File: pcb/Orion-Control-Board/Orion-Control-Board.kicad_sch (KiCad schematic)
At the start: 59 parts, among them J1 CONN_20_POS_KEYED_SOCKET, U1 BNO055, U2 INA3221, U3 DFR0753 5V BUCK, U4 PCA9685_PWM_SERVO_DRIVER_IC, U5 INA3221, U6 INA3221, Y1 32.768 kHz

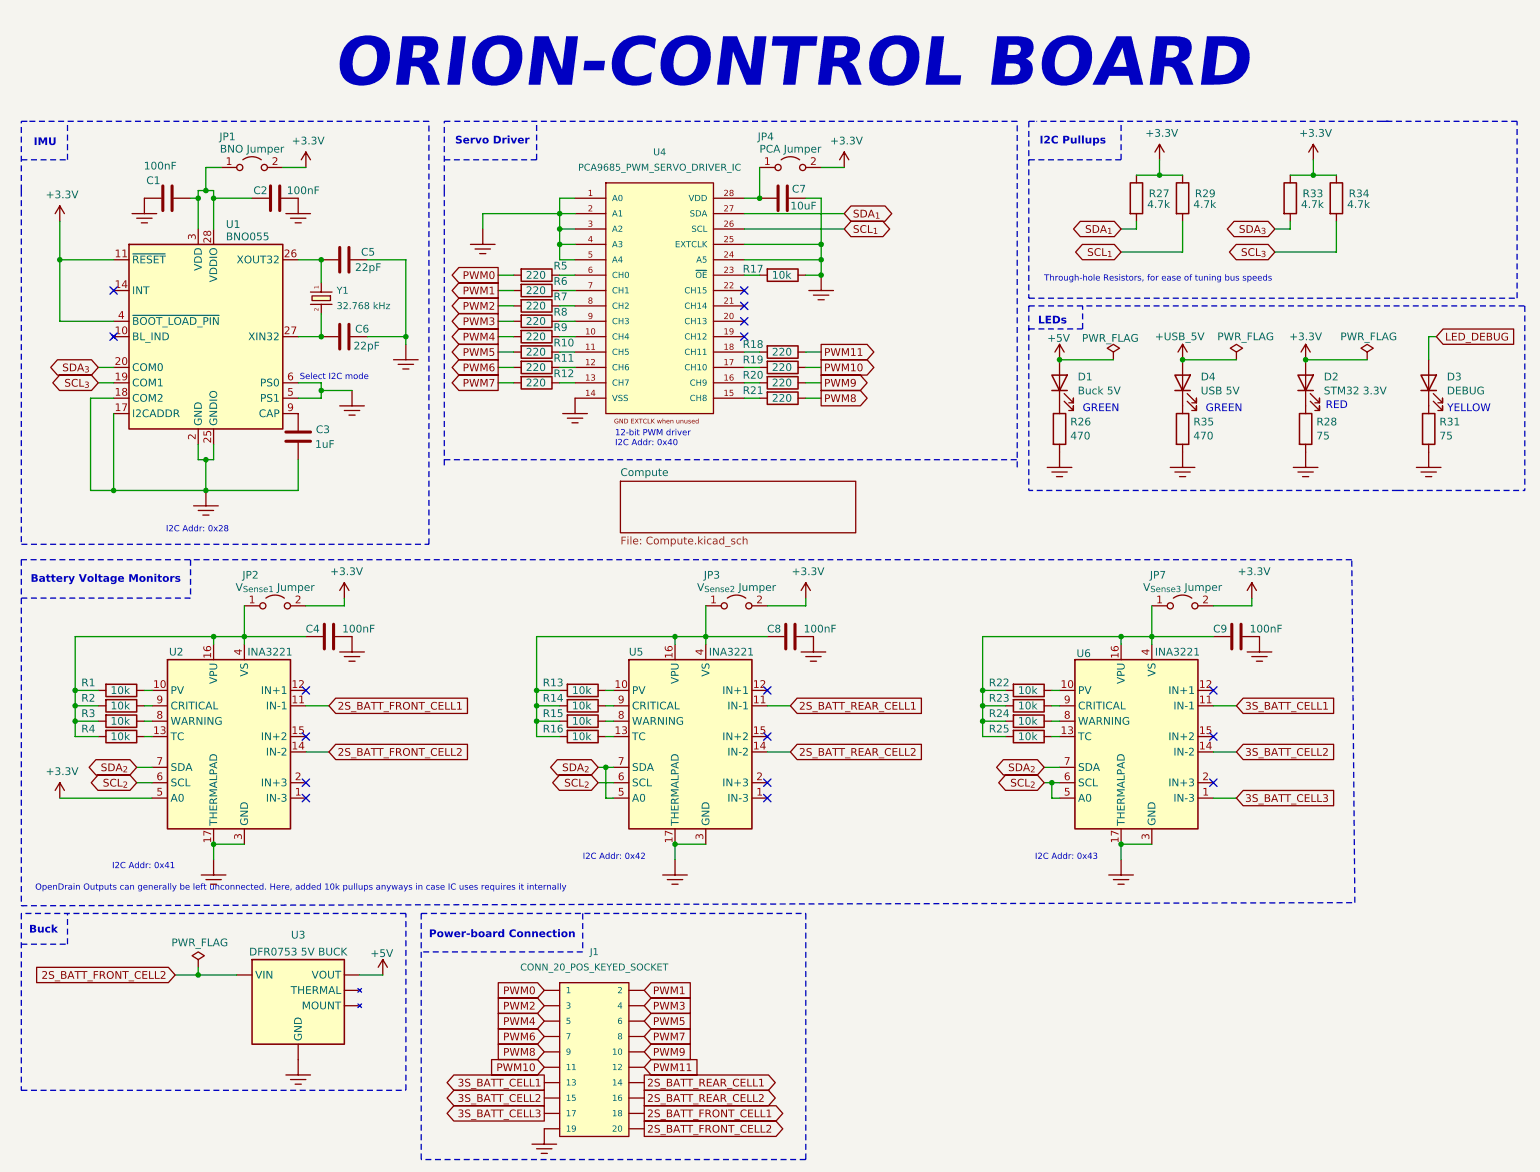
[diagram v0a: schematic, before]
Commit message: Update JLCPCB rules
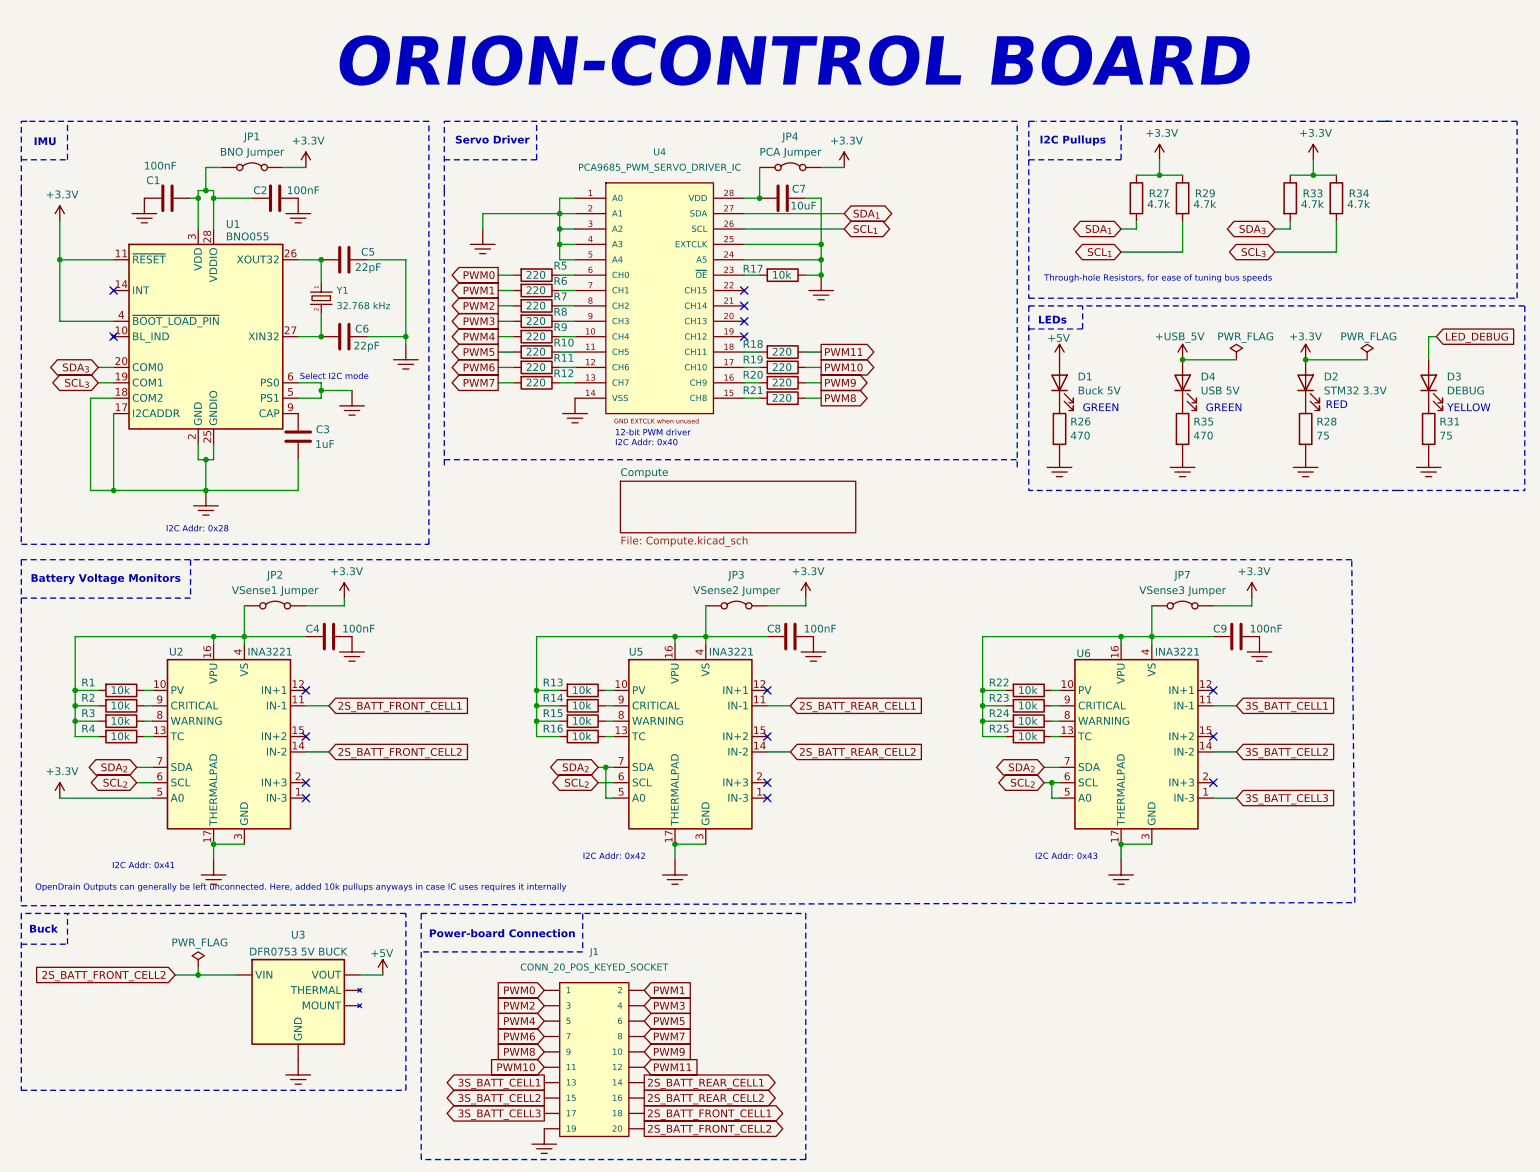
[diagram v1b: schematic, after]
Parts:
- removed JP1: BNO Jumper, AA_Custom_Components:Jumper_PinHeader_1x02_P2.54mm_Vertical, symbol Jumper:Jumper_2_Open
- removed JP2: V_{Sense1} Jumper, AA_Custom_Components:Jumper_PinHeader_1x02_P2.54mm_Vertical, symbol Jumper:Jumper_2_Open
- removed JP3: V_{Sense2} Jumper, AA_Custom_Components:Jumper_PinHeader_1x02_P2.54mm_Vertical, symbol Jumper:Jumper_2_Open
- removed JP4: PCA Jumper, AA_Custom_Components:Jumper_PinHeader_1x02_P2.54mm_Vertical, symbol Jumper:Jumper_2_Open
- removed JP7: V_{Sense3} Jumper, AA_Custom_Components:Jumper_PinHeader_1x02_P2.54mm_Vertical, symbol Jumper:Jumper_2_Open
- added JP1: BNO Jumper, AA_Custom_Components:Jumper_PinHeader_1x02_P2.54mm_Vertical, symbol Jumper:Jumper_2_Bridged
- added JP2: VSense1 Jumper, AA_Custom_Components:Jumper_PinHeader_1x02_P2.54mm_Vertical, symbol Jumper:Jumper_2_Bridged
- added JP3: VSense2 Jumper, AA_Custom_Components:Jumper_PinHeader_1x02_P2.54mm_Vertical, symbol Jumper:Jumper_2_Bridged
- added JP4: PCA Jumper, AA_Custom_Components:Jumper_PinHeader_1x02_P2.54mm_Vertical, symbol Jumper:Jumper_2_Bridged
- added JP7: VSense3 Jumper, AA_Custom_Components:Jumper_PinHeader_1x02_P2.54mm_Vertical, symbol Jumper:Jumper_2_Bridged
- Y1: footprint CRYSTAL-SMD-3.2X1.5MM -> Clocks:CRYSTAL-SMD-3.2X1.5MM
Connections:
- net +3.3V: now also JP1.2 (B), JP2.2 (B), JP3.2 (B), JP4.2 (B), JP7.2 (B)
- net at C8.1, R13.2, R14.2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: now also JP3.1 (A)
- net at C1.2, C2.1, U1.28 (VDDIO)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: now also JP1.1 (A)
- net at C9.1, R22.2, R23.2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: now also JP7.1 (A)
- net at C7.2, U4.28 (VDD): now also JP4.1 (A)
- net at C4.1, R1.2, R2.2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: now also JP2.1 (A)
